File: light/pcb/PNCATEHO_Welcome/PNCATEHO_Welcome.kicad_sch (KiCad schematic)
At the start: 61 parts, among them J1 USB_C_Receptacle_USB2.0, SW11 Boot, SW12 Reset, U1 RP2040, U2 RT9013-33GB, U3 W25Q32JVSSIQ, U4 USBLC6-2SC6, Y1 12MHz

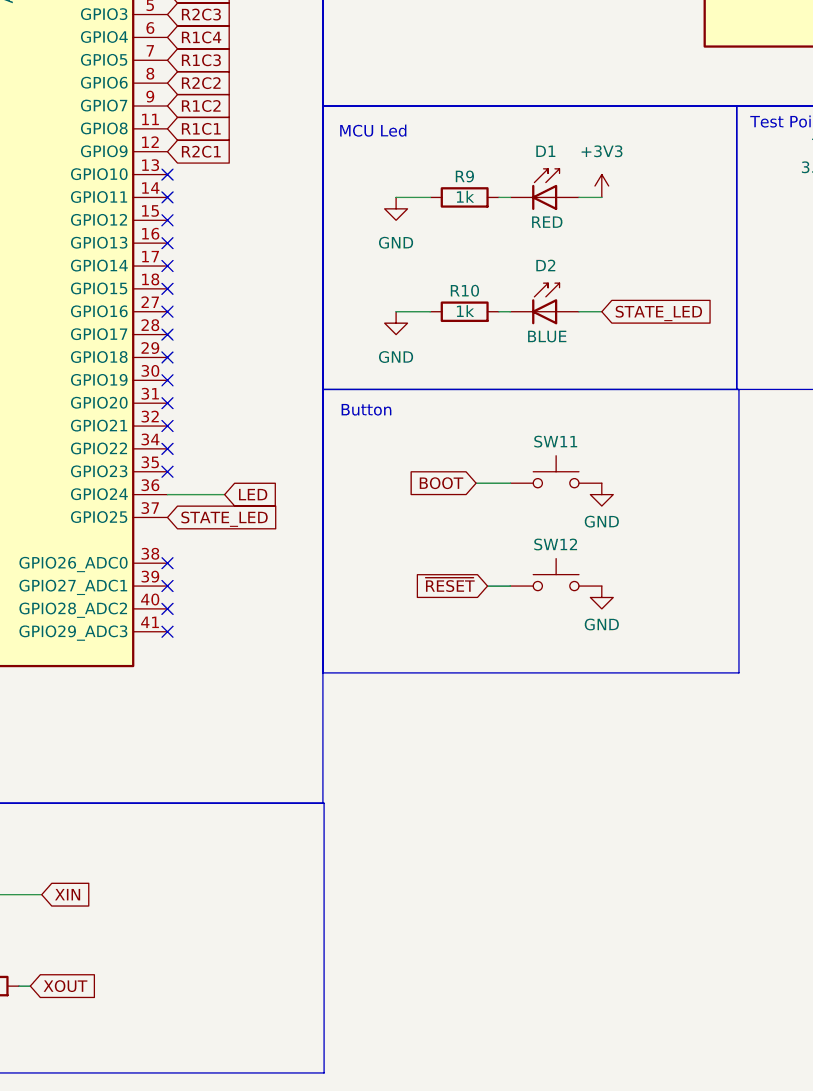
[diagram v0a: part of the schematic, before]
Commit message: update scheme
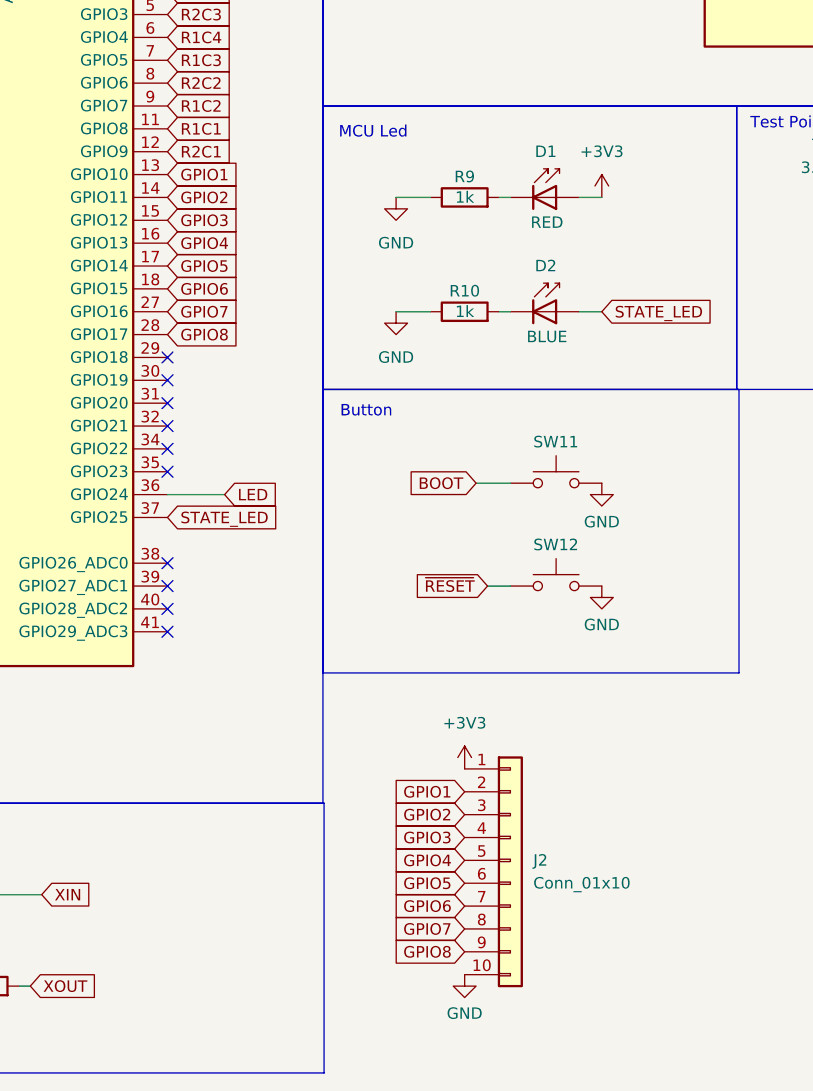
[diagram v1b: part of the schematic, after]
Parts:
- added J2: Conn_01x10, PNCATEHO:JST_GH_SM10B-GHS-TB_1x10-1MP_P1.25mm_Horizontal, symbol PNCATEHO:Conn_01x10
- U2: footprint PNCATEHO:SOT-23-5_L3.0-W1.7-P0.95-LS2.8-BL -> PNCATEHO:SOT-23-5_HandSoldering
- U4: footprint PNCATEHO:SOT-23-6_Handsoldering_REV -> PNCATEHO:SOT-23-6_Handsoldering
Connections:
- net +3V3: now also J2.1 (Pin_1)
- net GND: now also J2.10 (Pin_10)
- net GPIO1: now reaches U1.13 (GPIO10)
- net GPIO1: now also J2.2 (Pin_2)
- net GPIO2: now reaches U1.14 (GPIO11)
- net GPIO2: now also J2.3 (Pin_3)
- net GPIO3: now reaches U1.15 (GPIO12)
- net GPIO3: now also J2.4 (Pin_4)
- net GPIO4: now reaches U1.16 (GPIO13)
- net GPIO4: now also J2.5 (Pin_5)
- net GPIO5: now reaches U1.17 (GPIO14)
- net GPIO5: now also J2.6 (Pin_6)
- net GPIO6: now reaches U1.18 (GPIO15)
- net GPIO6: now also J2.7 (Pin_7)
- net GPIO7: now reaches U1.27 (GPIO16)
- net GPIO7: now also J2.8 (Pin_8)
- net GPIO8: now reaches U1.28 (GPIO17)
- net GPIO8: now also J2.9 (Pin_9)
- no-connect marks 21 -> 13

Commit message: update footprint
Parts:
- F1: footprint PNCATEHO:Fuse_0805_2012Metric -> PNCATEHO:Fuse_0805_2012Metric_Pad1.15x1.40mm_HandSolder
- TP1: footprint PNCATEHO:TestPoint_Pad_D2.0mm -> PNCATEHO:TestPoint_Pad_1.0x1.0mm
- TP2, TP3, TP4: footprint PNCATEHO:TestPoint_Pad_D2.0mm -> PNCATEHO:TestPoint_Pad_D1.0mm
- U1: footprint PNCATEHO:RP2040-QFN-56 -> PNCATEHO:QFN-56-1EP_7x7mm_P0.4mm_EP3.2x3.2mm_ThermalVias
- U3: footprint PNCATEHO:SOIC127P790X216-8N -> PNCATEHO:SOIC-8_5.3x5.3mm_P1.27mm
- Y1: footprint PNCATEHO:Crystal_SMD_3225-4Pin_3.2x2.5mm -> PNCATEHO:Crystal_SMD_3225-4Pin_3.2x2.5mm_HandSoldering
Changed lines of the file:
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@@
 			)
 		)
-		(property "Footprint" "PNCATEHO:TestPoint_Pad_D2.0mm"
+		(property "Footprint" "PNCATEHO:TestPoint_Pad_D1.0mm"
 			(at 185.42 137.16 0)
 			(effects
@@
 			)
 		)
-		(property "Footprint" "PNCATEHO:RP2040-QFN-56"
+		(property "Footprint" "PNCATEHO:QFN-56-1EP_7x7mm_P0.4mm_EP3.2x3.2mm_ThermalVias"
 			(at 60.96 129.54 0)
 			(effects
@@
 			)
 		)
-		(property "Footprint" "PNCATEHO:TestPoint_Pad_D2.0mm"
+		(property "Footprint" "PNCATEHO:TestPoint_Pad_1.0x1.0mm"
 			(at 166.37 137.16 0)
 			(effects
@@
 			)
 		)
-		(property "Footprint" "PNCATEHO:Fuse_0805_2012Metric"
+		(property "Footprint" "PNCATEHO:Fuse_0805_2012Metric_Pad1.15x1.40mm_HandSolder"
 			(at 54.61 24.13 0)
 			(effects
@@
 			)
 		)
-		(property "Footprint" "PNCATEHO:TestPoint_Pad_D2.0mm"
+		(property "Footprint" "PNCATEHO:TestPoint_Pad_D1.0mm"
 			(at 184.15 121.92 0)
 			(effects
@@
 			)
 		)
-		(property "Footprint" "PNCATEHO:Crystal_SMD_3225-4Pin_3.2x2.5mm"
+		(property "Footprint" "PNCATEHO:Crystal_SMD_3225-4Pin_3.2x2.5mm_HandSoldering"
 			(at 54.61 201.93 0)
 			(effects
@@
 			)
 		)
-		(property "Footprint" "PNCATEHO:SOIC127P790X216-8N"
+		(property "Footprint" "PNCATEHO:SOIC-8_5.3x5.3mm_P1.27mm"
 			(at 158.75 95.25 0)
 			(effects
@@
 			)
 		)
-		(property "Footprint" "PNCATEHO:TestPoint_Pad_D2.0mm"
+		(property "Footprint" "PNCATEHO:TestPoint_Pad_D1.0mm"
 			(at 165.1 121.92 0)
 			(effects

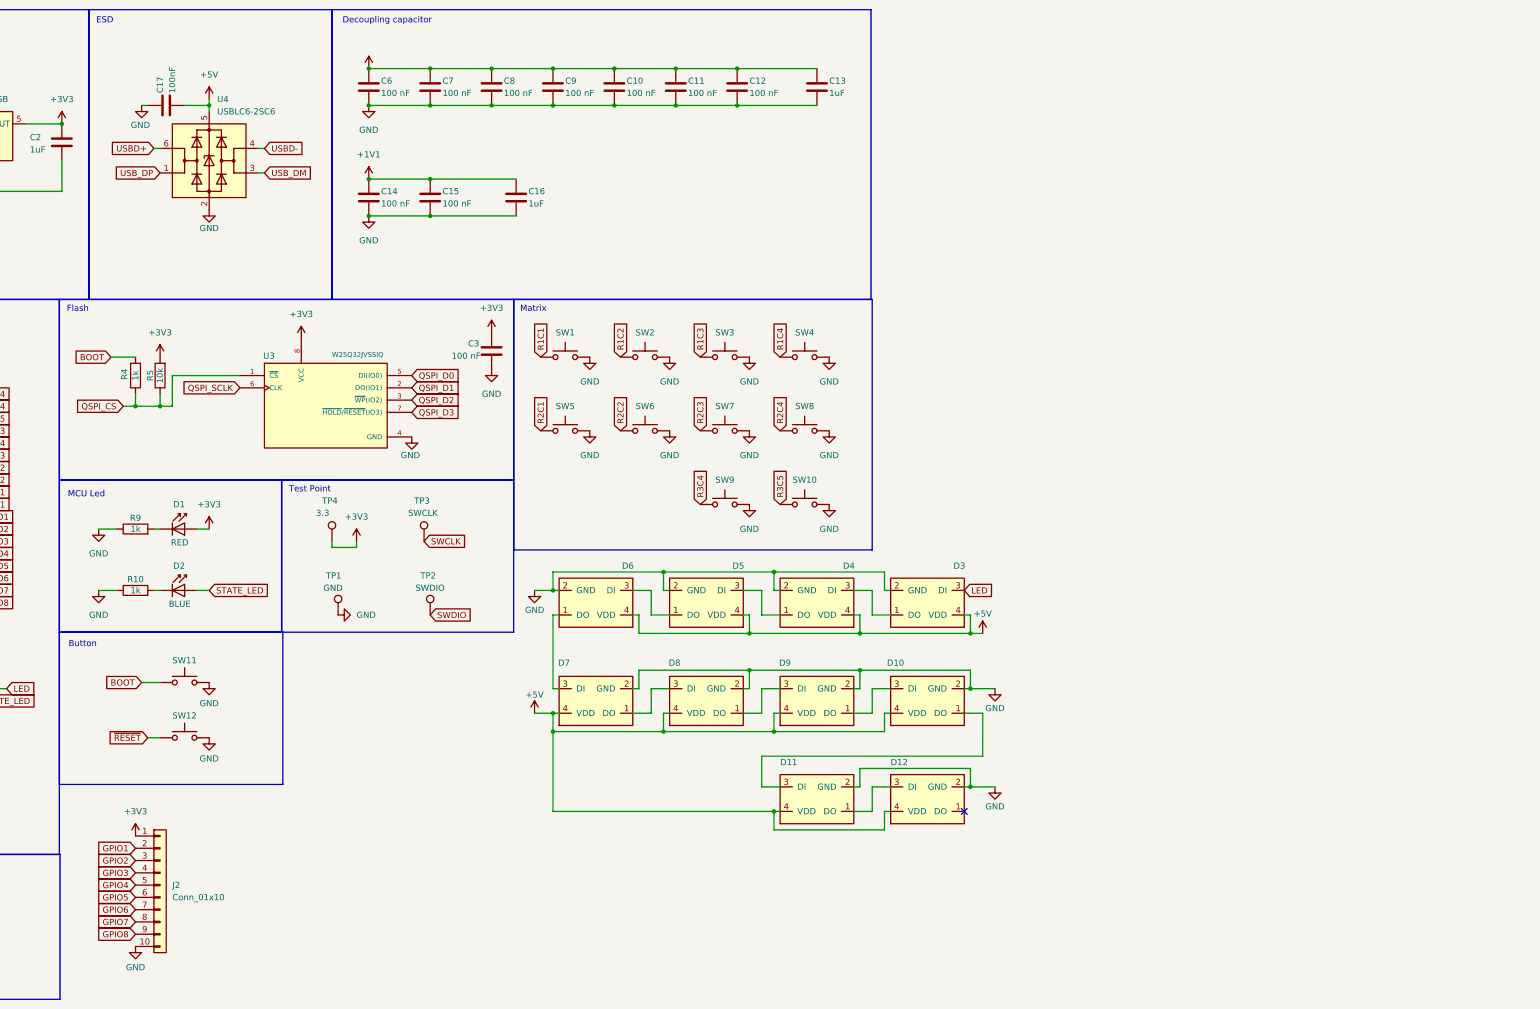
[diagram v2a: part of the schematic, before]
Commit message: update sh
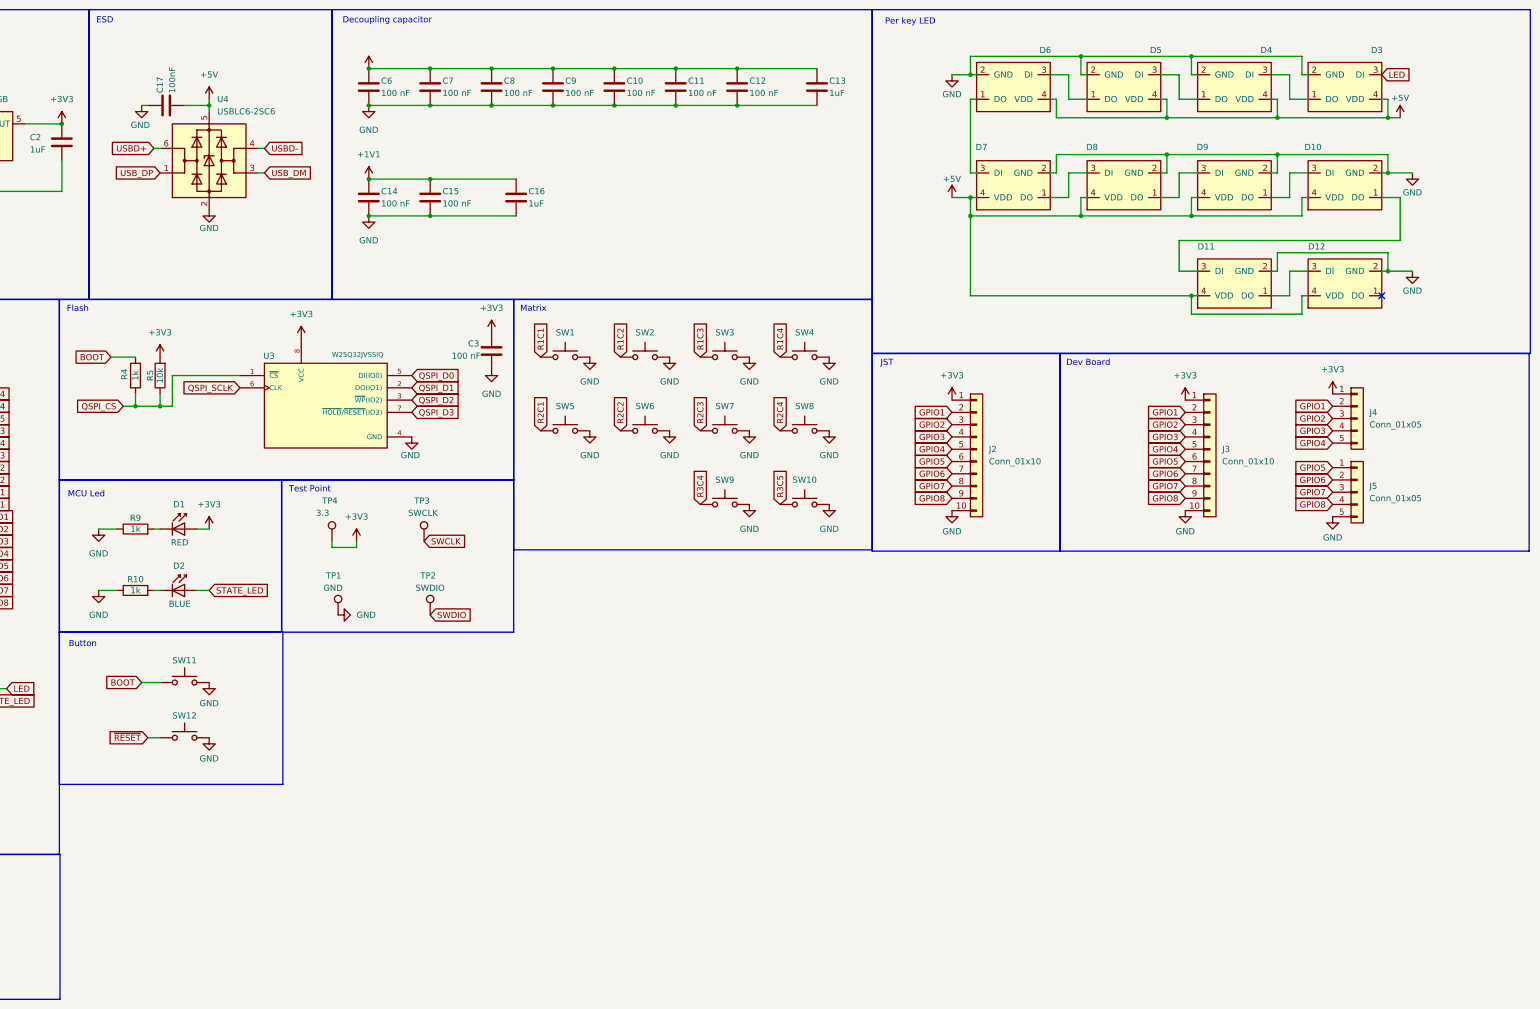
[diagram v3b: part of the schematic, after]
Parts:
- added J3: Conn_01x10, PNCATEHO:JST_GH_SM10B-GHS-TB_1x10-1MP_P1.25mm_Horizontal, symbol PNCATEHO:Conn_01x10
- added J4, J5: Conn_01x05, symbol PNCATEHO:Conn_01x05
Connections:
- net +3V3: now also J3.1 (Pin_1), J4.1 (Pin_1)
- net GND: now also J3.10 (Pin_10), J5.5 (Pin_5)
- net GPIO1: now also J3.2 (Pin_2), J4.2 (Pin_2)
- net GPIO2: now also J3.3 (Pin_3), J4.3 (Pin_3)
- net GPIO3: now also J3.4 (Pin_4), J4.4 (Pin_4)
- net GPIO4: now also J3.5 (Pin_5), J4.5 (Pin_5)
- net GPIO5: now also J3.6 (Pin_6), J5.1 (Pin_1)
- net GPIO6: now also J3.7 (Pin_7), J5.2 (Pin_2)
- net GPIO7: now also J3.8 (Pin_8), J5.3 (Pin_3)
- net GPIO8: now also J3.9 (Pin_9), J5.4 (Pin_4)
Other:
- note added: "Dev Board"
- note added: "JST"
- note added: "Per key LED"
- moved on the sheet: D10, D11, D12, D3, D4, D5, D6, D7, D8, D9, J2
